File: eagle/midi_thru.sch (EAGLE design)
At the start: 25 parts, among them IC2 40106N

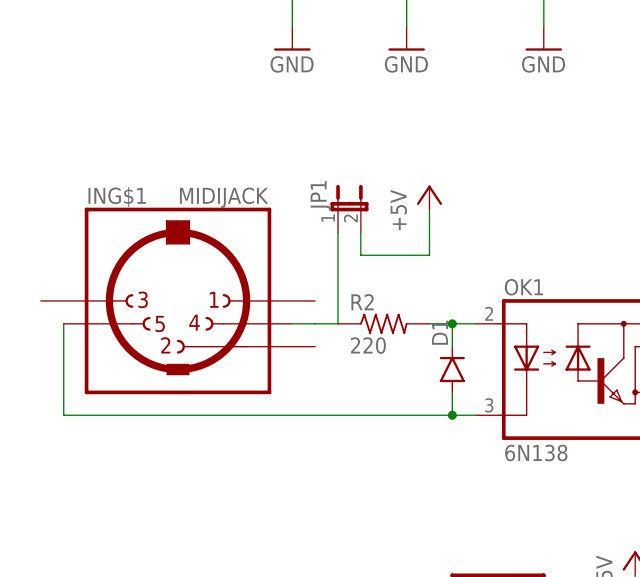
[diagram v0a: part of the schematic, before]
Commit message: first cut happened
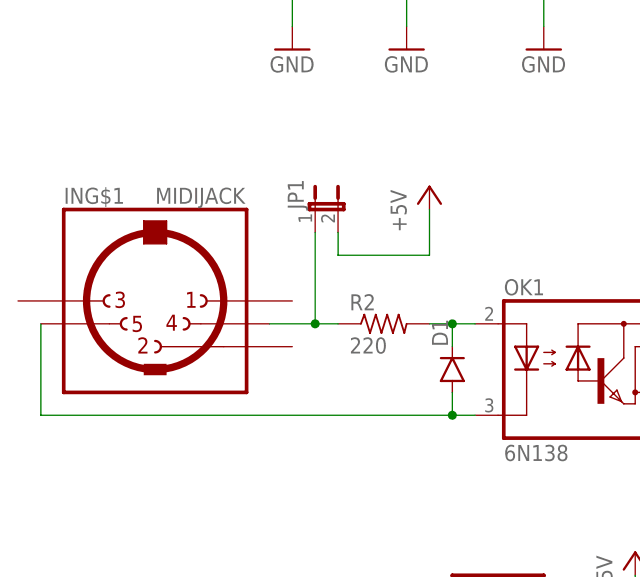
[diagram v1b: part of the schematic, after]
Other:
- moved on the sheet: ING$1, JP1
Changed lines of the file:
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@@
 <instance part="THRU_3" gate="G$1" x="162.56" y="93.98"/>
 <instance part="THRU_4" gate="G$1" x="162.56" y="71.12"/>
-<instance part="IN" gate="G$1" x="12.7" y="114.3"/>
-<instance part="JP1" gate="A" x="30.48" y="124.46"/>
+<instance part="IN" gate="G$1" x="10.16" y="114.3"/>
+<instance part="JP1" gate="A" x="27.94" y="124.46"/>
 <instance part="P+3" gate="1" x="40.64" y="127"/>
 <instance part="THRU_1" gate="G$2" x="38.1" y="157.48"/>
@@
 <junction x="43.18" y="101.6"/>
 <pinref part="IN" gate="G$1" pin="5"/>
-<wire x1="0" y1="111.76" x2="0" y2="101.6" width="0.1524" layer="91"/>
-<wire x1="0" y1="101.6" x2="43.18" y2="101.6" width="0.1524" layer="91"/>
+<wire x1="-2.54" y1="111.76" x2="-2.54" y2="101.6" width="0.1524" layer="91"/>
+<wire x1="-2.54" y1="101.6" x2="43.18" y2="101.6" width="0.1524" layer="91"/>
 </segment>
 </net>
@@
 <segment>
 <pinref part="JP1" gate="A" pin="2"/>
-<wire x1="33.02" y1="121.92" x2="33.02" y2="119.38" width="0.1524" layer="91"/>
+<wire x1="30.48" y1="121.92" x2="30.48" y2="119.38" width="0.1524" layer="91"/>
 <pinref part="P+3" gate="1" pin="+5V"/>
-<wire x1="33.02" y1="119.38" x2="40.64" y2="119.38" width="0.1524" layer="91"/>
+<wire x1="30.48" y1="119.38" x2="40.64" y2="119.38" width="0.1524" layer="91"/>
 <wire x1="40.64" y1="119.38" x2="40.64" y2="124.46" width="0.1524" layer="91"/>
 </segment>
@@
 <pinref part="R2" gate="G$1" pin="1"/>
 <pinref part="IN" gate="G$1" pin="4"/>
+<wire x1="22.86" y1="111.76" x2="27.94" y2="111.76" width="0.1524" layer="91"/>
 <pinref part="JP1" gate="A" pin="1"/>
-<wire x1="27.94" y1="111.76" x2="25.4" y2="111.76" width="0.1524" layer="91"/>
 <wire x1="27.94" y1="111.76" x2="30.48" y2="111.76" width="0.1524" layer="91"/>
-<wire x1="30.48" y1="111.76" x2="30.48" y2="121.92" width="0.1524" layer="91"/>
+<wire x1="27.94" y1="121.92" x2="27.94" y2="111.76" width="0.1524" layer="91"/>
+<junction x="27.94" y="111.76"/>
 </segment>
 </net>
@@
 </sheet>
 </sheets>
+<errors>
+</errors>
 </schematic>
 </drawing>
